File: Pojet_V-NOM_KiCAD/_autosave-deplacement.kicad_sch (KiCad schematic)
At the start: 8 parts, among them J301 Conn_01x06, J302 Conn_01x06, U301 ZXBM5210-SP, U302 ZXBM5210-SP

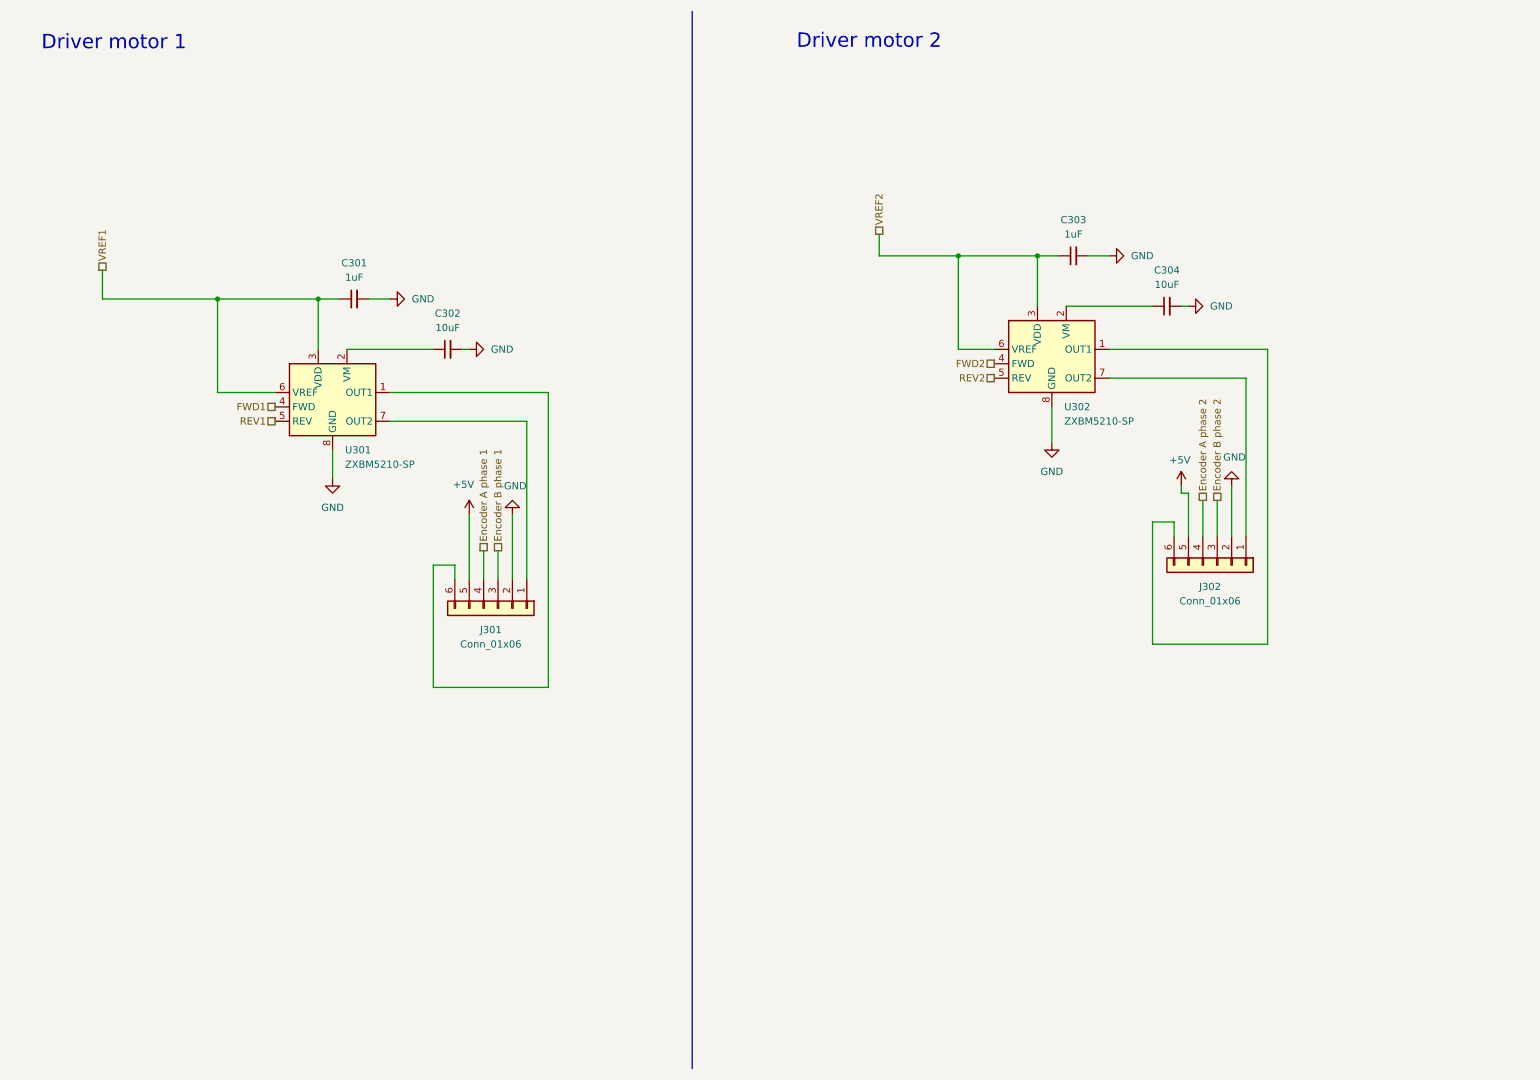
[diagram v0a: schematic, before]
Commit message: DEPLACEMENT
maj Deplacement
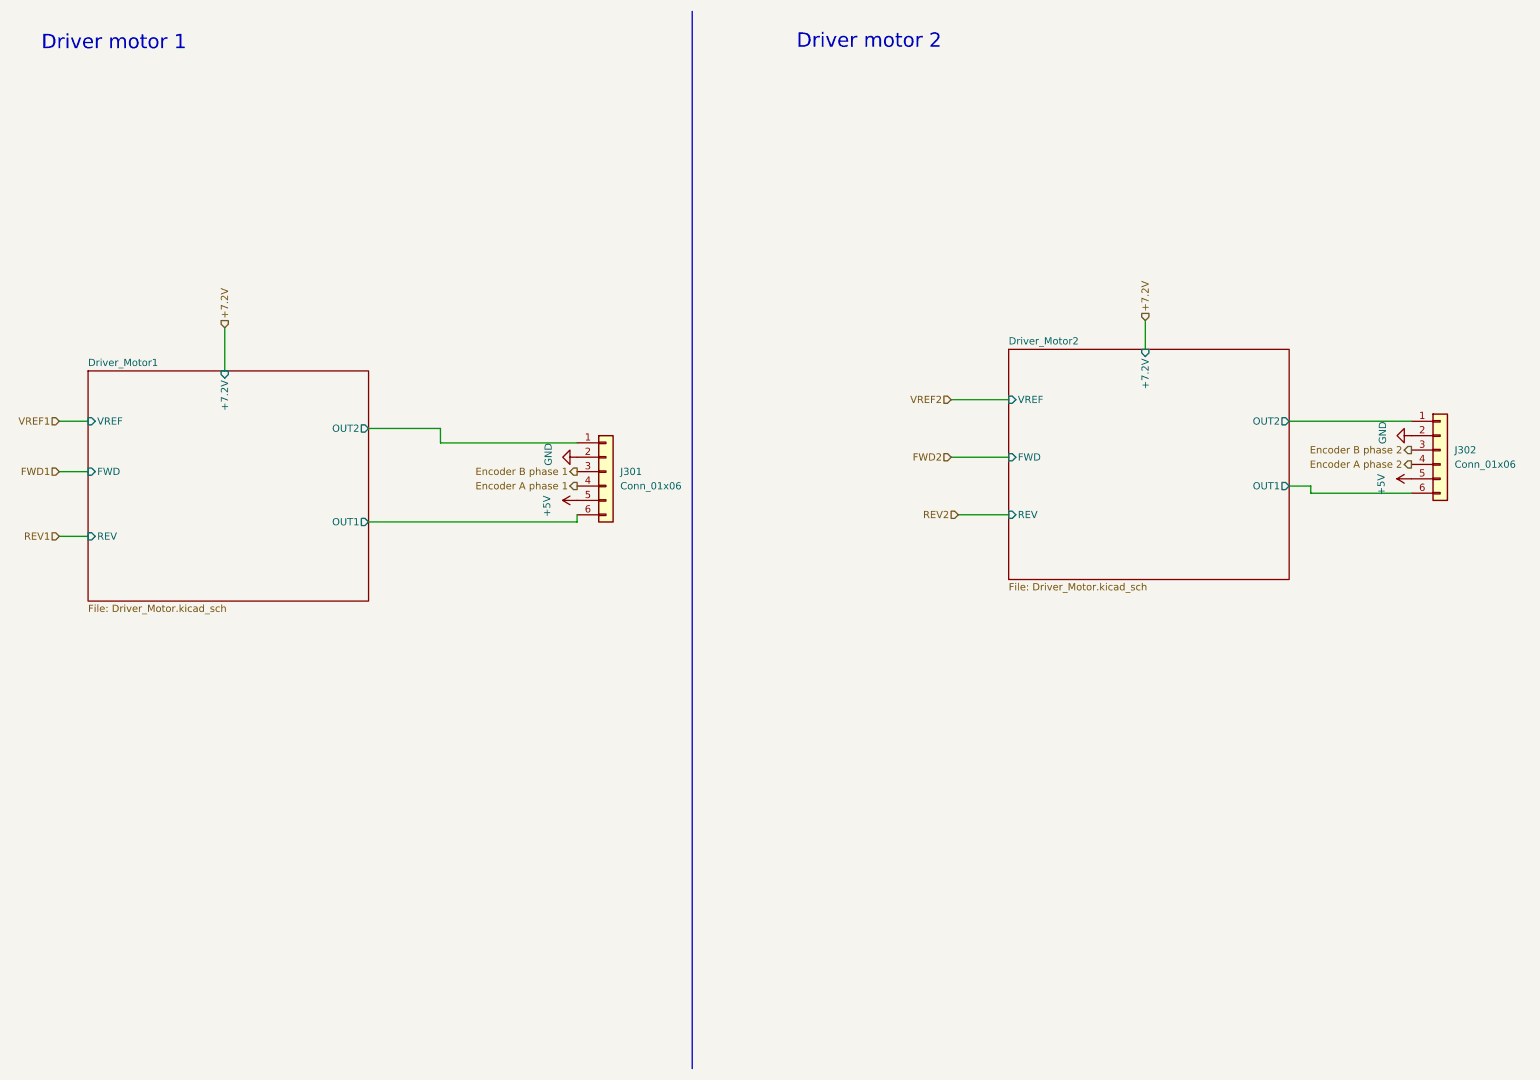
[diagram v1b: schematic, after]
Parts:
- removed C301, C303: 1uF, Capacitor_SMD:C_0402_1005Metric, symbol Device:C_Small
- removed C302, C304: 10uF, Capacitor_SMD:C_0402_1005Metric, symbol Device:C_Small
- removed U301, U302: ZXBM5210-SP, Package_SO:Diodes_SO-8EP, symbol Driver_Motor:ZXBM5210-SP
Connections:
- net Driver_Motor1/OUT1: now reaches J301.6 (Pin_6)
- net Driver_Motor1/OUT2: now reaches J301.1 (Pin_1)
- net Driver_Motor2/OUT2: now reaches J302.1 (Pin_1)
- net Driver_Motor2/OUT1: now reaches J302.6 (Pin_6)
- net Encoder A phase 1  renamed Encoder A phase 1
- net Encoder B phase 1  renamed Encoder B phase 1
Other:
- added sheet Driver_Motor1 (Driver_Motor.kicad_sch)
- added sheet Driver_Motor2 (Driver_Motor.kicad_sch)
